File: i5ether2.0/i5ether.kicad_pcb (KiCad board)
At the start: 2 copper layers, 90.2 x 31.2 mm, 14 parts, among them J2 Conn_02x05_Odd_Even, J3 1-406541-1, T2 HX5008

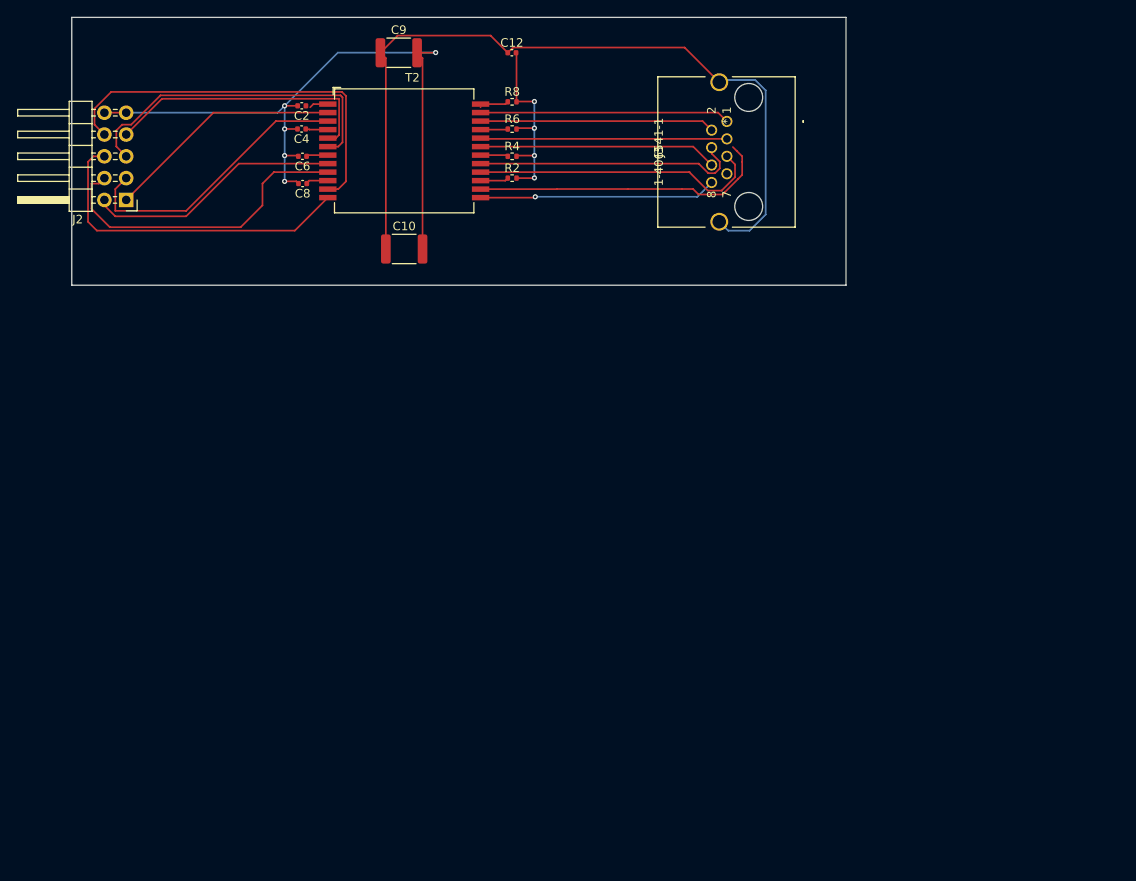
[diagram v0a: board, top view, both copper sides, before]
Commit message: Avances en placa
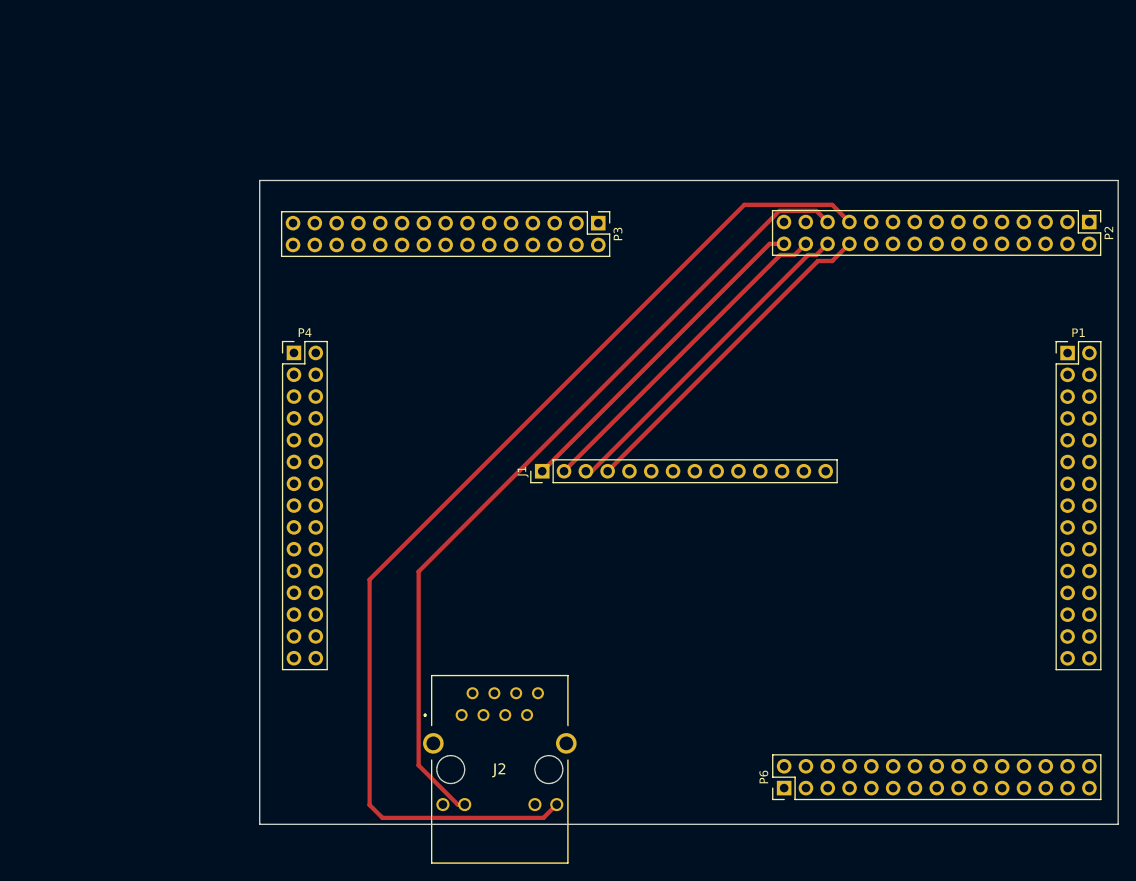
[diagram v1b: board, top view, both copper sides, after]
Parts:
- removed C10, C9: 4700p, Resistor_SMD:R_1812_4532Metric
- removed C12: 1000p, Capacitor_SMD:C_0402_1005Metric
- removed C2, C4, C6, C8: 0.1u, Capacitor_SMD:C_0402_1005Metric
- removed J3: 1-406541-1, MJ406541:1-406541-1
- removed R2, R4, R6, R8: 75, Resistor_SMD:R_0402_1005Metric
- removed T2: HX5008, HX5008:HX5008NL
- added J1: Conn_01x14, Connector_PinHeader_2.54mm:PinHeader_1x14_P2.54mm_Vertical, F.Cu at (126.9, 109.9)
- added P1: Conn_02x15_Counter_Clockwise, Connector_PinHeader_2.54mm:PinHeader_2x15_P2.54mm_Vertical, F.Cu at (188.1, 96.1)
- added P2: Conn_02x15_Counter_Clockwise, Connector_PinHeader_2.54mm:PinHeader_2x15_P2.54mm_Vertical, F.Cu at (190.6, 80.8)
- added P3: Conn_02x15_Counter_Clockwise, Connector_PinHeader_2.54mm:PinHeader_2x15_P2.54mm_Vertical, F.Cu at (133.4, 81.0)
- added P4: Conn_02x15_Counter_Clockwise, Connector_PinHeader_2.54mm:PinHeader_2x15_P2.54mm_Vertical, F.Cu at (98.0, 96.1)
- added P6: Conn_02x15_Counter_Clockwise, Connector_PinHeader_2.54mm:PinHeader_2x15_P2.54mm_Vertical, F.Cu at (155.1, 146.8)
- J2: value Conn_02x05_Odd_Even -> 7499011121A; footprint Connector_PinHeader_2.54mm:PinHeader_2x05_P2.54mm_Horizontal -> KiCad:7499011121A
- moved J2 79.3 mm to (122.0, 144.6)
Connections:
- J2 pad 1: Net-(J2-Pin_1) -> /ethernet_module/TD+
- J2 pad 10: GND -> /ethernet_module/YLED-
- J2 pad 2: Net-(J2-Pin_2) -> +3.3V
- J2 pad 3: Net-(J2-Pin_3) -> /ethernet_module/TD-
- J2 pad 4: Net-(J2-Pin_4) -> /ethernet_module/RD+
- J2 pad 5: Net-(J2-Pin_5) -> +3.3V
- J2 pad 6: Net-(J2-Pin_6) -> /ethernet_module/RD-
- J2 pad 7: Net-(J2-Pin_7) -> unconnected-(J2-Pad7)
- J2 pad 8: Net-(J2-Pin_8) -> unconnected-(J2-Pad8)
- J2 pad 9: GND -> +3.3V
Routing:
- net /ethernet_module/GLED-: track 0.00 -> 124.1 mm
- net /ethernet_module/YLED-: track 0.00 -> 95.4 mm
- net Earth: track 93.4 -> 0.00 mm
- net GND: track 82.1 -> 0.00 mm, vias 5 -> 0
- net Net-(J2-Pin_8): track 46.2 -> 0.00 mm
- net /screen_module/T_DO: track 0.00 -> 39.1 mm
- net /screen_module/T_IRQ: track 0.00 -> 39.1 mm
- net /screen_module/T_DIN: track 0.00 -> 39.1 mm
- net /screen_module/T_CS: track 0.00 -> 39.1 mm
- net Net-(J2-Pin_6): track 39.1 -> 0.00 mm
- net Net-(J2-Pin_5): track 39.0 -> 0.00 mm
- net Net-(J2-Pin_4): track 37.3 -> 0.00 mm
- net Net-(T2-MX4+): track 35.4 -> 0.00 mm
- net Net-(T2-MX3-): track 34.0 -> 0.00 mm
- net Net-(J2-Pin_3): track 33.4 -> 0.00 mm
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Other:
- board size 90.2 x 31.2 mm -> 100 x 75 mm
- rule pad_to_mask_clearance: 0.051 -> 0
